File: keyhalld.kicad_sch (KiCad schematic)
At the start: 42 parts, among them J1 Conn_ARM_SWD_TagConnect_TC203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, J2 USB_C_Receptacle_USB2.0_16P, J3 Conn_01x05_Pin, U1 AMS1117-3.3, U2 USBLC6-2SC6, U3 RP2350A, U4 CD74HC4067M, Y1 12MHz

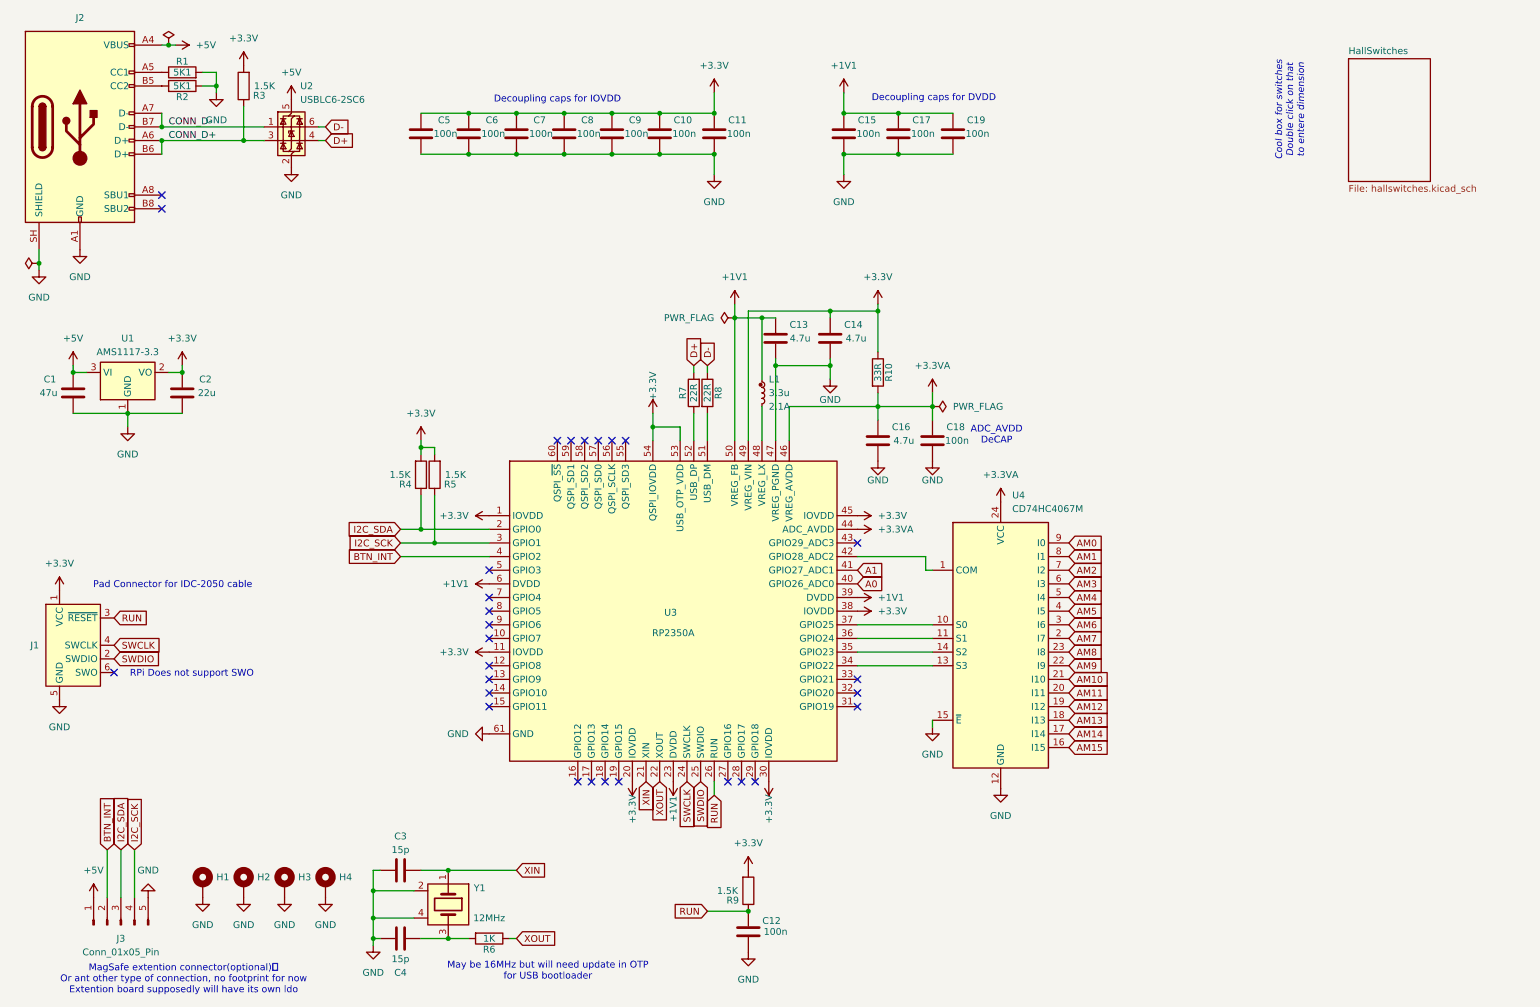
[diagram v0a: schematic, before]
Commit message: Modularize sheets. Still WIP
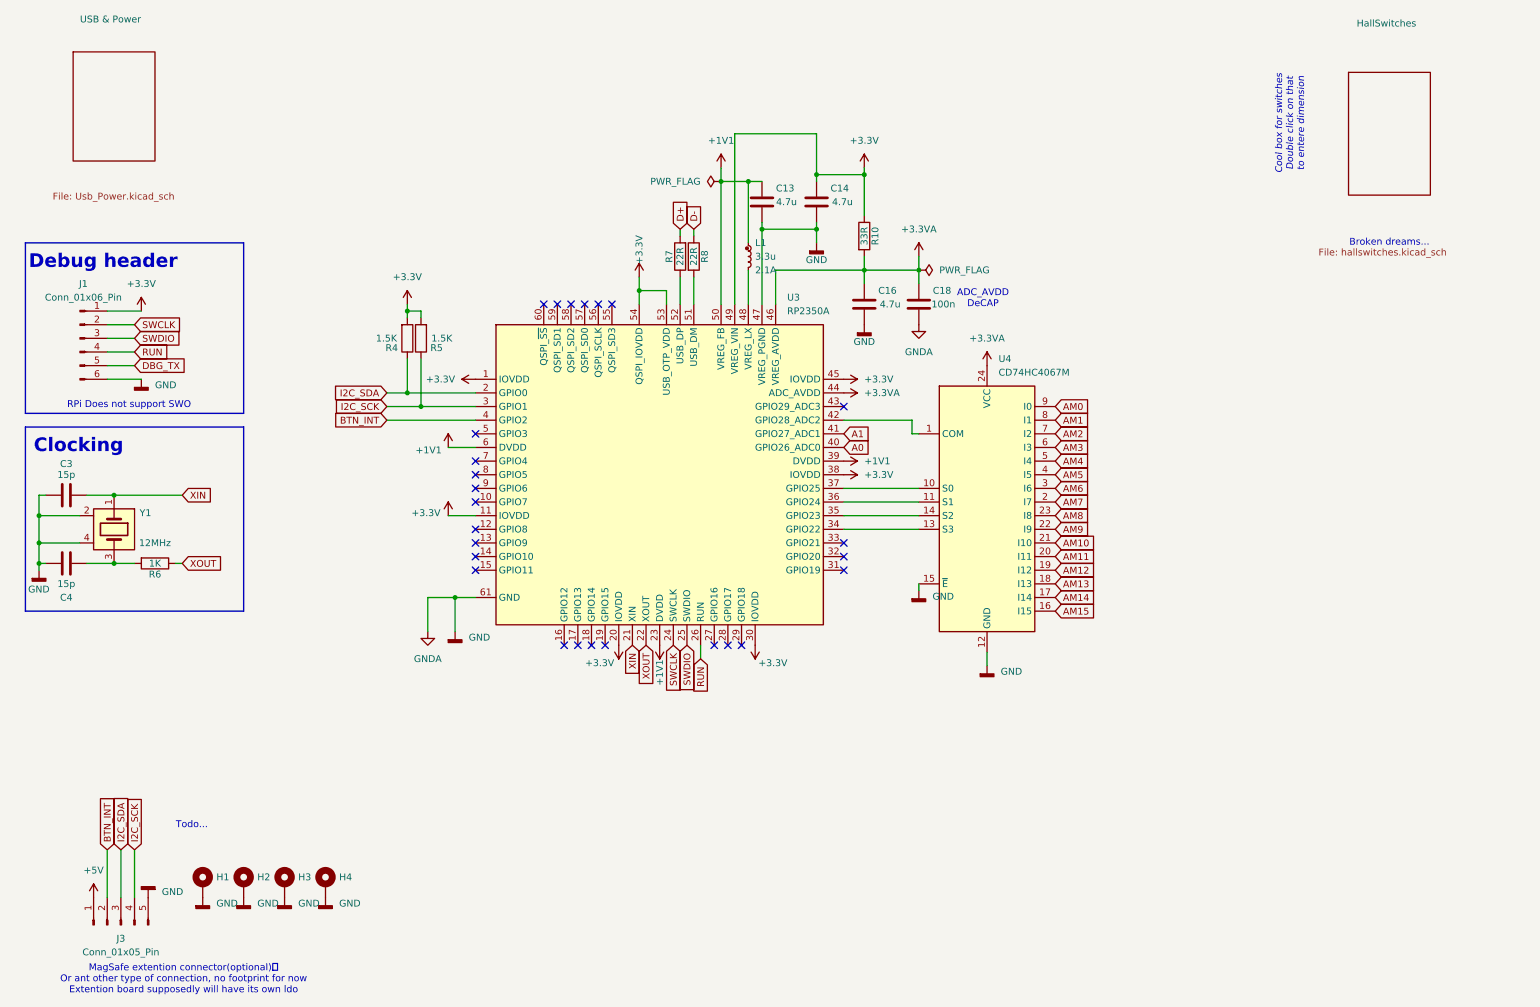
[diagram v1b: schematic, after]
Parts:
- removed C1: 47u, Capacitor_SMD:C_0603_1608Metric_Pad1.08x0.95mm_HandSolder, symbol Device:C
- removed C10, C11, C12, C15, C17, C19, C5, C6, C7, C8, C9: 100n, Capacitor_SMD:C_0603_1608Metric_Pad1.08x0.95mm_HandSolder, symbol Device:C
- removed C2: 22u, Capacitor_SMD:C_0603_1608Metric_Pad1.08x0.95mm_HandSolder, symbol Device:C
- removed J1: Conn_ARM_SWD_TagConnect_TC2030-NL, Connector:Tag-Connect_TC2030-IDC-NL_2x03_P1.27mm_Vertical, symbol Connector:Conn_ARM_SWD_TagConnect_TC2030-NL
- removed J2: USB_C_Receptacle_USB2.0_16P, Connector_USB:USB_C_Receptacle_GCT_USB4105-xx-A_16P_TopMnt_Horizontal, symbol Connector:USB_C_Receptacle_USB2.0_16P
- removed R1, R2: 5K1, Resistor_SMD:R_0603_1608Metric_Pad0.98x0.95mm_HandSolder, symbol Device:R
- removed R3, R9: 1.5K, Resistor_SMD:R_0603_1608Metric_Pad0.98x0.95mm_HandSolder, symbol Device:R
- removed U1: AMS1117-3.3, Package_TO_SOT_SMD:SOT-223-3_TabPin2, symbol Regulator_Linear:AMS1117-3.3
- removed U2: USBLC6-2SC6, Package_TO_SOT_SMD:SOT-23-6, symbol Power_Protection:USBLC6-2SC6
- added J1: Conn_01x06_Pin, Connector_PinHeader_1.00mm:PinHeader_1x06_P1.00mm_Vertical, symbol Connector:Conn_01x06_Pin
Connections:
- net +3.3V: now also J1.1 (Pin_1)
- net GND: now also J1.6 (Pin_6)
- net RUN: now also J1.4 (Pin_4)
- net SWCLK: now also J1.2 (Pin_2)
- net SWDIO: now also J1.3 (Pin_3)
- new net DBG_TX: J1.5 (Pin_5)
- no-connect marks 29 -> 26
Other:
- added sheet USB & Power (Usb_Power.kicad_sch)
- note added: "Broken dreams..."
- note added: "Clocking"
- note added: "Debug header"
- note added: "Todo..."
- note removed: "Decoupling caps for DVDD"
- note removed: "Decoupling caps for IOVDD"
- note removed: "May be 16MHz but will need update in OTP for USB bootloader"
- note removed: "Pad Connector for IDC-2050 cable"
- title: Magnetic Keyboard with Hall sensors -> Magnetic Keyboard with Hall sensors (MCU)
- moved on the sheet: C13, C14, C16, C18, C3, C4, L1, R10, R4, R5, R6, R7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
